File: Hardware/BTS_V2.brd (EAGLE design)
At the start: 113 x 79.4 mm, 63 parts, among them IC1 TPA3140D2PWP, IC2 BLK-MD-SPK-B, J1 SPKR_OUT, J2 RN52BoB_R, J3 RN52BoB_L, J4 TFT_CONNECTION, J6 HC-05, T3_2 TEENSY_3.1-3.2_DIL

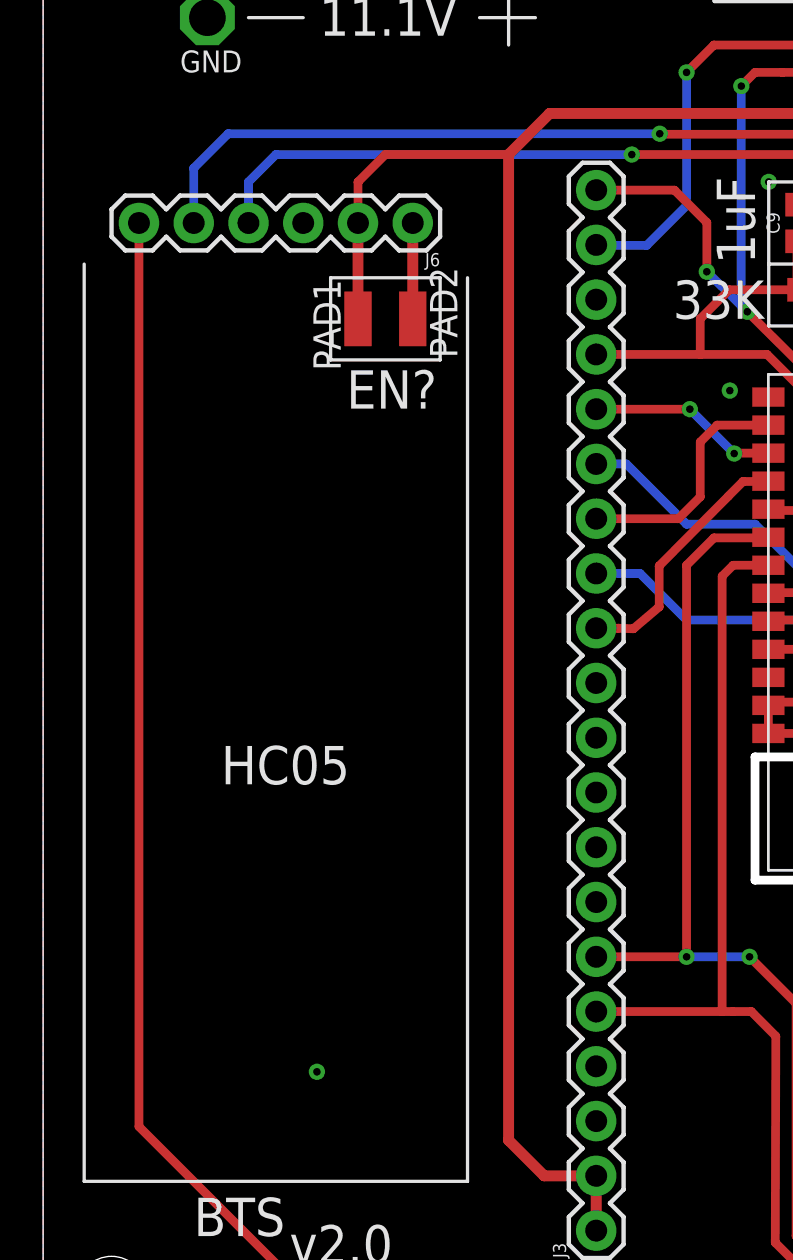
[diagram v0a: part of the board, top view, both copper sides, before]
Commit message: Further error fixed
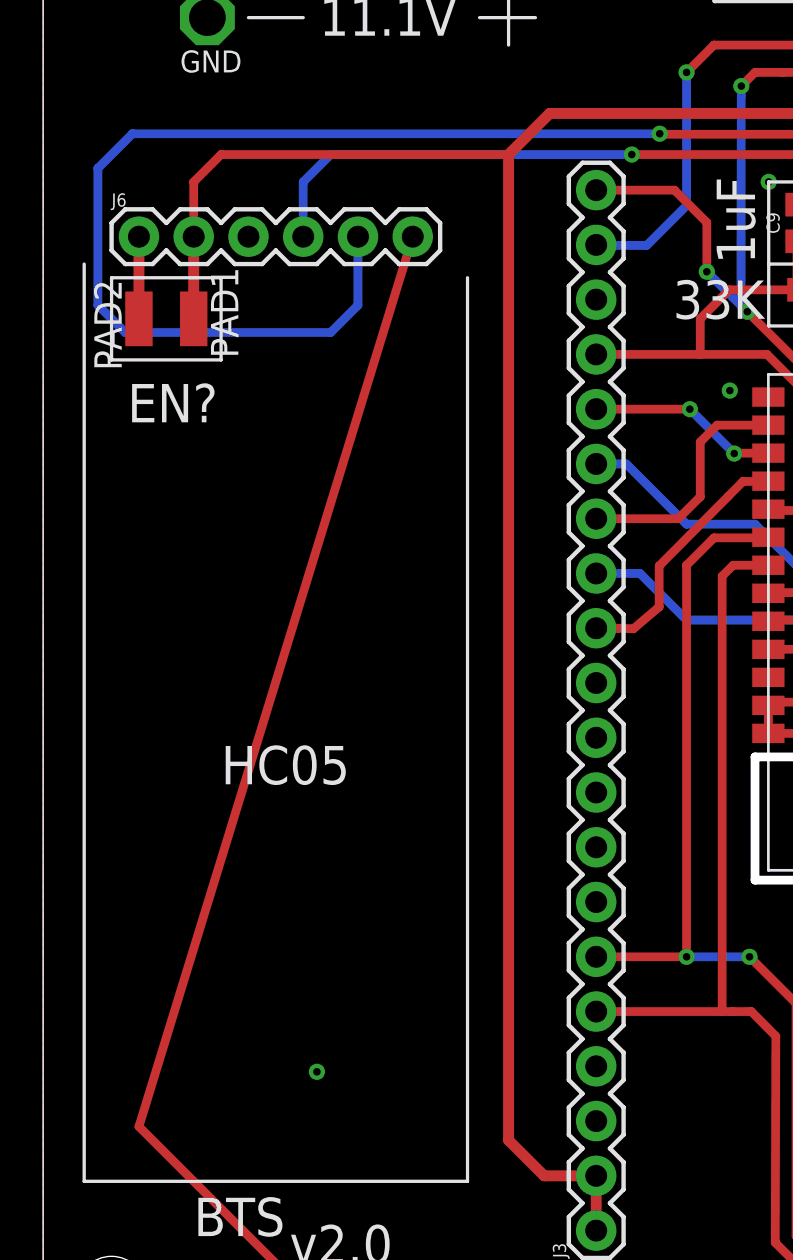
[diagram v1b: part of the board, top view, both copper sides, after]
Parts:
- moved J6 12.7 mm to (4.45, 52.1), turned to 0 degrees
- moved PAD2 12.7 mm to (4.45, 48.3), turned to 0 degrees
- moved PAD1 7.62 mm to (6.99, 48.3), turned to 180 degrees
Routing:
- net HC_UART_RX: track 132.8 -> 157.4 mm
- net 3V3: track 250.2 -> 257.8 mm
- net HC_UART_TX: track 123.1 -> 121.2 mm
- net STATE: track 148.0 -> 149.3 mm
- net EN: track 4.45 -> 3.81 mm
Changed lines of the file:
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@@
 <wire x1="68.58" y1="14.3002" x2="68.58" y2="12.319" width="0.1524" layer="21"/>
 <wire x1="72.39" y1="14.3002" x2="72.39" y2="12.319" width="0.1524" layer="21"/>
-<text x="14.0716" y="44.0944" size="1.778" layer="21" font="vector">EN?</text>
+<text x="3.9116" y="43.4594" size="1.778" layer="21" font="vector">EN?</text>
 <wire x1="66.04" y1="42.926" x2="69.85" y2="42.926" width="0.1524" layer="21"/>
 <wire x1="69.85" y1="42.926" x2="69.85" y2="40.9448" width="0.1524" layer="21"/>
@@
 <wire x1="78.8162" y1="24.0284" x2="78.105" y2="24.0284" width="0.1524" layer="21"/>
 <wire x1="68.5038" y1="24.0284" x2="69.1896" y2="24.0284" width="0.1524" layer="21"/>
-<wire x1="13.335" y1="50.165" x2="18.415" y2="50.165" width="0.1524" layer="21"/>
-<wire x1="18.415" y1="50.165" x2="18.415" y2="46.355" width="0.1524" layer="21"/>
-<wire x1="18.415" y1="46.355" x2="13.335" y2="46.355" width="0.1524" layer="21"/>
-<wire x1="13.335" y1="46.355" x2="13.335" y2="50.165" width="0.1524" layer="21"/>
+<wire x1="8.255" y1="46.355" x2="3.175" y2="46.355" width="0.1524" layer="21"/>
+<wire x1="3.175" y1="46.355" x2="3.175" y2="50.165" width="0.1524" layer="21"/>
+<wire x1="3.175" y1="50.165" x2="8.255" y2="50.165" width="0.1524" layer="21"/>
+<wire x1="8.255" y1="50.165" x2="8.255" y2="46.355" width="0.1524" layer="21"/>
 <text x="22.225" y="1.905" size="1.778" layer="21" font="vector">RN52L</text>
 <text x="52.07" y="1.905" size="1.778" layer="21" font="vector">RN52R</text>
@@
 <attribute name="RESISTANCE" value="10K" x="55.499" y="63.8302" size="1.778" layer="27" rot="R180" display="off"/>
 </element>
-<element name="J6" library="SparkFun-Connectors" library_urn="urn:adsk.eagle:library:513" package="1X06" package3d_urn="urn:adsk.eagle:package:38009/1" value="HC-05" x="17.145" y="52.705" rot="R180">
-<attribute name="PROD_ID" value="CONN-08437" x="17.145" y="52.705" size="1.778" layer="27" rot="R180" display="off"/>
-</element>
-<element name="PAD1" library="wirepad" library_urn="urn:adsk.eagle:library:412" package="SMD1,27-2,54" package3d_urn="urn:adsk.eagle:package:30839/1" value="?" x="14.605" y="48.26"/>
-<element name="PAD2" library="wirepad" library_urn="urn:adsk.eagle:library:412" package="SMD1,27-2,54" package3d_urn="urn:adsk.eagle:package:30839/1" value="?" x="17.145" y="48.26" rot="R180"/>
+<element name="J6" library="SparkFun-Connectors" library_urn="urn:adsk.eagle:library:513" package="1X06" package3d_urn="urn:adsk.eagle:package:38009/1" value="HC-05" x="4.445" y="52.07">
+<attribute name="PROD_ID" value="CONN-08437" x="4.445" y="52.07" size="1.778" layer="27" display="off"/>
+</element>
+<element name="PAD1" library="wirepad" library_urn="urn:adsk.eagle:library:412" package="SMD1,27-2,54" package3d_urn="urn:adsk.eagle:package:30839/1" value="?" x="6.985" y="48.26" rot="R180"/>
+<element name="PAD2" library="wirepad" library_urn="urn:adsk.eagle:library:412" package="SMD1,27-2,54" package3d_urn="urn:adsk.eagle:package:30839/1" value="?" x="4.445" y="48.26"/>
 <element name="T3_2" library="Teensy_3_and_LC_Series_Boards_v1.4" package="TEENSY_3.0-3.2&amp;LC_DIL" value="TEENSY_3.1-3.2_DIL" x="92.71" y="22.225"/>
 <element name="R15" library="resistor" library_urn="urn:adsk.eagle:library:348" package="R0603" package3d_urn="urn:adsk.eagle:package:26057/1" value="10K" x="78.74" y="33.655" rot="R180">
@@
 <contactref element="J3" pad="1"/>
 <wire x1="39.37" y1="57.785" x2="23.495" y2="57.785" width="0.508" layer="1"/>
-<wire x1="14.605" y1="48.26" x2="14.605" y2="52.705" width="0.508" layer="1"/>
+<wire x1="6.985" y1="48.26" x2="6.985" y2="52.07" width="0.508" layer="1"/>
 <wire x1="23.495" y1="57.785" x2="21.59" y2="55.88" width="0.508" layer="1"/>
 <wire x1="21.59" y1="55.88" x2="21.59" y2="10.16" width="0.508" layer="1"/>
@@
 <via x="85.3694" y="46.355" extent="1-16" drill="0.35"/>
 <wire x1="85.3694" y1="46.355" x2="90.17" y2="46.355" width="0.508" layer="1"/>
-<wire x1="14.605" y1="52.705" x2="14.605" y2="54.61" width="0.4064" layer="1"/>
-<wire x1="14.605" y1="54.61" x2="15.875" y2="55.88" width="0.4064" layer="1"/>
-<wire x1="15.875" y1="55.88" x2="21.59" y2="55.88" width="0.4064" layer="1"/>
 <via x="81.28" y="46.355" extent="1-16" drill="0.35"/>
 <wire x1="62.865" y1="60.53" x2="62.865" y2="60.325" width="0.4064" layer="1"/>
@@
 <wire x1="73.9394" y1="48.2854" x2="73.914" y2="48.26" width="0.508" layer="1"/>
 <wire x1="73.914" y1="48.26" x2="72.006" y2="48.26" width="0.508" layer="1"/>
+<wire x1="8.255" y1="55.88" x2="6.985" y2="54.61" width="0.4064" layer="1"/>
+<wire x1="6.985" y1="54.61" x2="6.985" y2="52.07" width="0.4064" layer="1"/>
+<wire x1="21.59" y1="55.88" x2="8.255" y2="55.88" width="0.4064" layer="1"/>
 </signal>
 <signal name="N$65">
@@
 <wire x1="87.63" y1="8.89" x2="87.63" y2="14.605" width="0.4064" layer="16"/>
 <via x="87.63" y="14.605" extent="1-16" drill="0.35"/>
-<wire x1="4.445" y1="10.795" x2="4.445" y2="52.705" width="0.4064" layer="1"/>
+<wire x1="4.445" y1="10.795" x2="17.145" y2="52.07" width="0.4064" layer="1"/>
 <wire x1="87.63" y1="14.605" x2="87.63" y2="19.685" width="0.4064" layer="1"/>
 <wire x1="87.63" y1="19.685" x2="86.36" y2="20.955" width="0.4064" layer="1"/>
@@
 <contactref element="J6" pad="1"/>
 <contactref element="PAD2" pad="1"/>
-<wire x1="17.145" y1="48.26" x2="17.145" y2="52.705" width="0.508" layer="1"/>
+<wire x1="4.445" y1="48.26" x2="4.445" y2="52.07" width="0.508" layer="1"/>
 </signal>
 <signal name="HC_UART_TX">
@@
 <wire x1="89.535" y1="14.605" x2="88.265" y2="13.335" width="0.4064" layer="1"/>
 <wire x1="88.265" y1="13.335" x2="85.09" y2="13.335" width="0.4064" layer="1"/>
-<wire x1="9.525" y1="52.705" x2="9.525" y2="54.61" width="0.4064" layer="16"/>
-<wire x1="9.525" y1="54.61" x2="10.795" y2="55.88" width="0.4064" layer="16"/>
-<wire x1="10.795" y1="55.88" x2="27.305" y2="55.88" width="0.4064" layer="16"/>
+<wire x1="13.335" y1="55.88" x2="27.305" y2="55.88" width="0.4064" layer="16"/>
 <wire x1="85.3948" y1="43.815" x2="81.28" y2="43.815" width="0.4064" layer="16"/>
 <via x="81.28" y="43.815" extent="1-16" drill="0.35"/>
@@
 <wire x1="89.535" y1="41.275" x2="86.995" y2="43.815" width="0.4064" layer="1"/>
 <wire x1="86.995" y1="43.815" x2="85.3948" y2="43.815" width="0.4064" layer="1"/>
+<wire x1="12.065" y1="52.07" x2="12.065" y2="54.61" width="0.4064" layer="16"/>
+<wire x1="12.065" y1="54.61" x2="13.335" y2="55.88" width="0.4064" layer="16"/>
 </signal>
 <signal name="HC_UART_RX">
@@
 <wire x1="38.1" y1="56.8198" x2="28.6258" y2="56.8198" width="0.4064" layer="1"/>
 <wire x1="28.6258" y1="56.8198" x2="28.6004" y2="56.8452" width="0.4064" layer="1"/>
-<wire x1="6.985" y1="52.705" x2="6.985" y2="55.245" width="0.4064" layer="16"/>
-<wire x1="6.985" y1="55.245" x2="8.5852" y2="56.8452" width="0.4064" layer="16"/>
-<wire x1="8.5852" y1="56.8452" x2="28.6004" y2="56.8452" width="0.4064" layer="16"/>
+<wire x1="4.1402" y1="56.8452" x2="28.6004" y2="56.8452" width="0.4064" layer="16"/>
 <wire x1="88.265" y1="10.795" x2="90.805" y2="13.335" width="0.4064" layer="1"/>
 <via x="79.375" y="45.085" extent="1-16" drill="0.35"/>
@@
 <wire x1="90.805" y1="13.335" x2="90.805" y2="43.815" width="0.4064" layer="1"/>
 <wire x1="90.805" y1="43.815" x2="89.535" y2="45.085" width="0.4064" layer="1"/>
+<wire x1="4.1402" y1="56.8452" x2="2.54" y2="55.245" width="0.4064" layer="16"/>
+<wire x1="2.54" y1="55.245" x2="2.54" y2="48.895" width="0.4064" layer="16"/>
+<wire x1="2.54" y1="48.895" x2="3.81" y2="47.625" width="0.4064" layer="16"/>
+<wire x1="3.81" y1="47.625" x2="13.335" y2="47.625" width="0.4064" layer="16"/>
+<wire x1="13.335" y1="47.625" x2="14.605" y2="48.895" width="0.4064" layer="16"/>
+<wire x1="14.605" y1="48.895" x2="14.605" y2="52.07" width="0.4064" layer="16"/>
 </signal>
 <signal name="N$25">
